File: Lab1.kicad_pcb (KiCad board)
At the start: 2 copper layers, 60 x 40 mm, 49 parts, among them J1 USB_OTG, J2 SWD, SW2 Reset, U1 PMW3389, U2 AP2125N-3.3TRG, U3 MIC5235YM5-TR, U4 STM32F411RETx, U5 USBLC6-2SC6, Y1 16Mhz

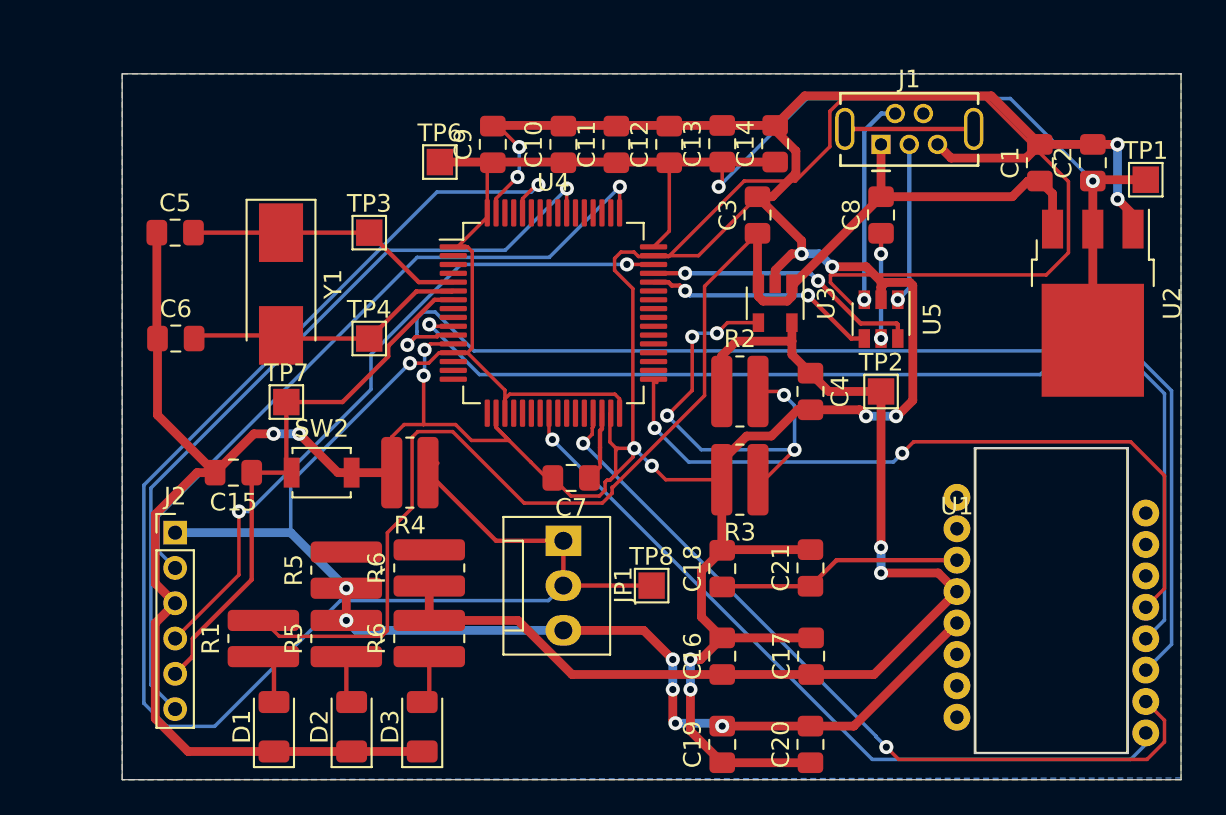
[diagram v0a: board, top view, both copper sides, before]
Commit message: 2nd design, quite happy with this one!
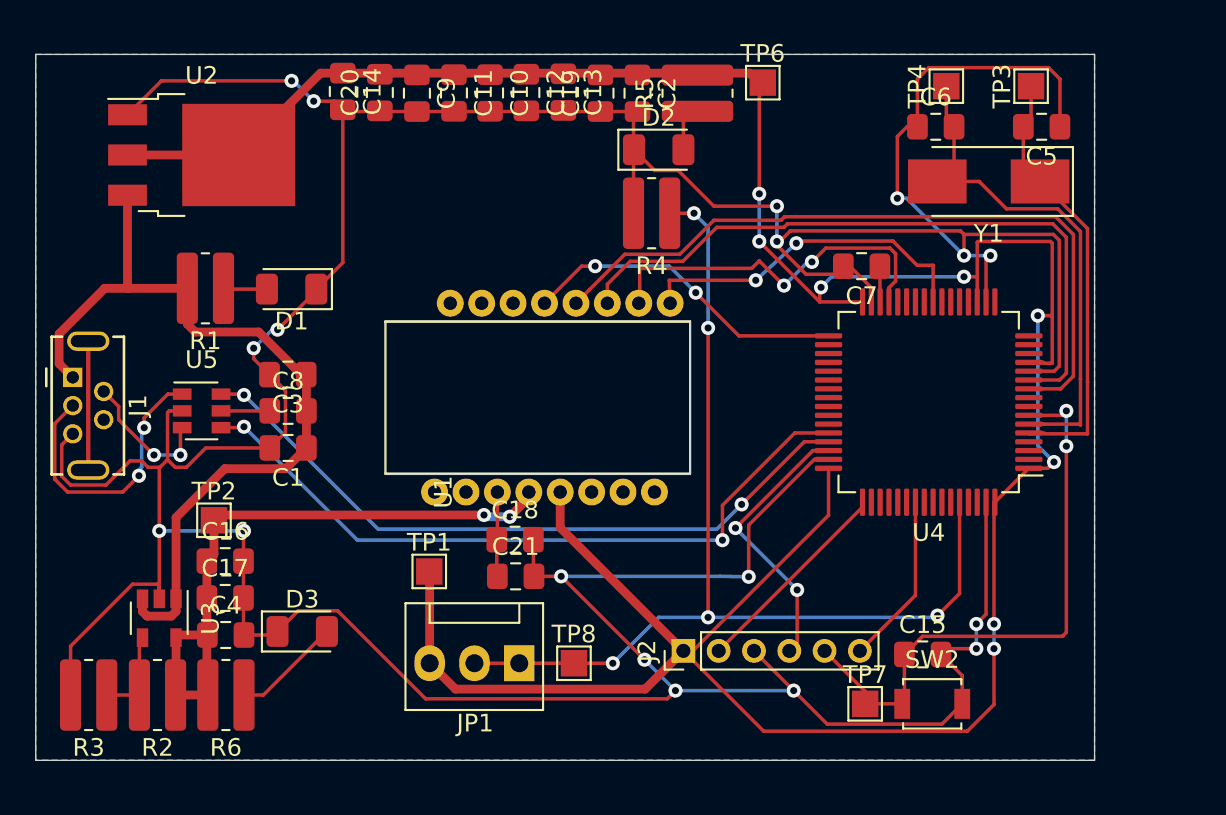
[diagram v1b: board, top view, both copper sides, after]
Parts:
- removed the R5 at (61.7, 59.1)
- removed the R5 at (61.7, 63.0)
- removed the R6 at (66.4, 59.0)
- removed the R6 at (66.4, 63.0)
- added R5: 820, Resistor_SMD:R_0815_2038Metric_Pad1.20x4.05mm_HandSolder, F.Cu at (81.6, 32.1)
- added R6: 47, Resistor_SMD:R_0815_2038Metric_Pad1.20x4.05mm_HandSolder, F.Cu at (54.9, 66.2)
- moved U2 51.2 mm to (53.5, 35.6), turned to 0 degrees
- moved C5 49.5 mm to (101.1, 34.0), turned to 180 degrees
- moved J1 47.7 mm to (46.2, 48.2), turned to 270 degrees
- moved TP1 46.3 mm to (66.4, 59.2)
- moved C1 45.6 mm to (58.4, 52.2), turned to 180 degrees
- moved C6 44.7 mm to (95.1, 34.0)
- moved C20 44.3 mm to (63.6, 32.1)
- moved Y1 40.5 mm to (98.1, 37.1), turned to 180 degrees
- moved C15 40.4 mm to (94.4, 63.9), turned to 0 degrees
- moved U3 39.2 mm to (51.1, 61.9)
- moved R3 38.9 mm to (47.1, 66.2)
- moved U5 38.8 mm to (53.5, 50.1), turned to 0 degrees
- moved TP2 38.5 mm to (54.2, 56.3)
- moved TP3 38.4 mm to (100.5, 31.7), turned to 90 degrees
- moved C19 37.5 mm to (76.1, 32.1)
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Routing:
- net SWO: track 45.1 -> 9.73 mm, vias 1 -> 0
- net +5V: track 79.5 -> 47.7 mm
- net BOOT0: track 89.0 -> 58.9 mm, vias 2 -> 5
- net MOSI: track 68.1 -> 38.8 mm, vias 1 -> 0
- net VDD: track 64.2 -> 35.8 mm
- net OUT_D-: track 13.3 -> 40.8 mm
- net SWCLK: track 38.7 -> 11.8 mm, vias 2 -> 0
- net GND: track 301.1 -> 274.9 mm, vias 16 -> 18
- net SCK: track 45.5 -> 21.2 mm, vias 3 -> 2
- net Motion: track 43.7 -> 19.8 mm, vias 1 -> 2
- net OUT_D+: track 15.8 -> 39.6 mm
- net SWDIO: track 39.2 -> 15.7 mm
- net NCS: track 41.9 -> 18.6 mm
- net MISO: track 61.2 -> 41.5 mm, vias 2 -> 0
- net Net-(R2-Pad2): track 24.8 -> 5.17 mm, vias 5 -> 0
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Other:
- outline, holes or cut-outs redrawn
